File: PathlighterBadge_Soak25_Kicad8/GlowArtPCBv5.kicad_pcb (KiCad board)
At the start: 2 copper layers, 93.2 x 113.9 mm, 13 parts, among them SW1 SW_SPDT

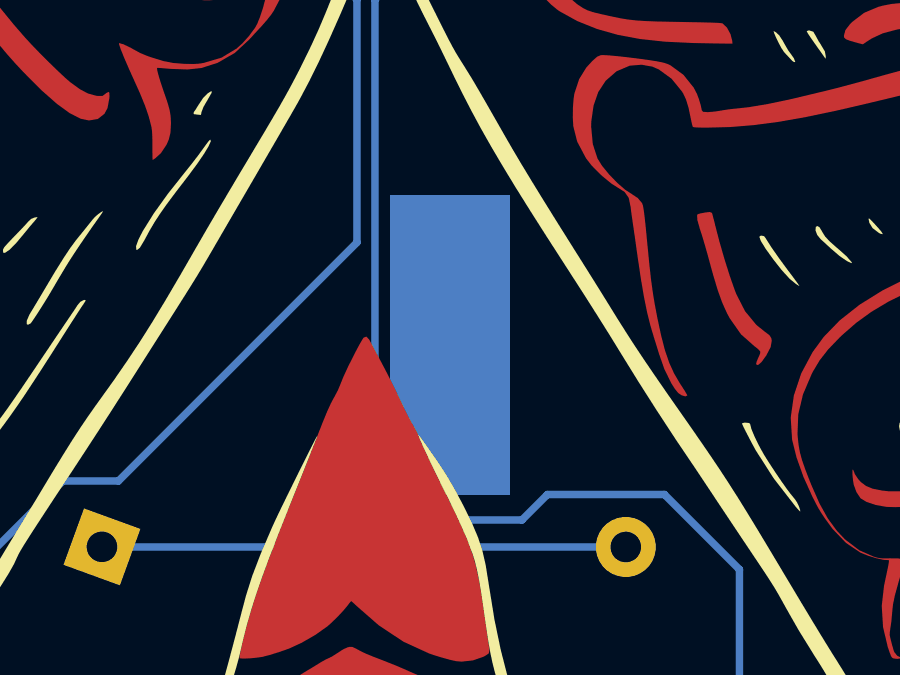
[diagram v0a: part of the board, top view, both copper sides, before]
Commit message: Rework backbone
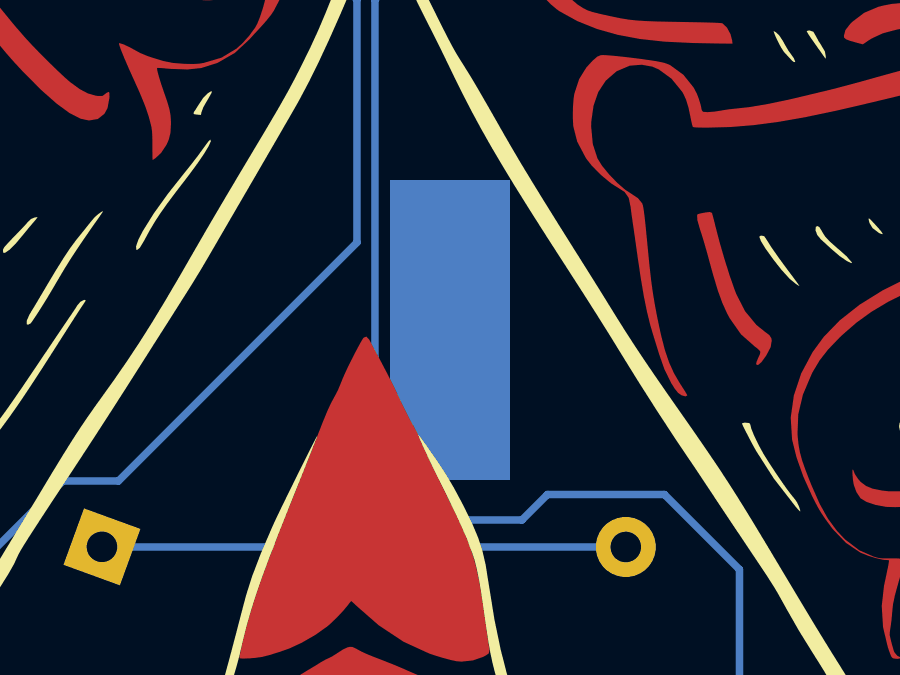
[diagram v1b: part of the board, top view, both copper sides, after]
